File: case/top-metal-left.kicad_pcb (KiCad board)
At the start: 2 copper layers, 134.3 x 93.7 mm, 25 parts, among them SW1 SW_PUSH, SW10 SW_PUSH, SW11 SW_PUSH, SW12 SW_PUSH, SW13 SW_PUSH, SW14 SW_PUSH, SW15 SW_PUSH, SW16 SW_PUSH, SW17 SW_PUSH, SW18 SW_PUSH, SW19 SW_PUSH, SW2 SW_PUSH, SW20 SW_PUSH, SW3 SW_PUSH, SW4 SW_PUSH, SW5 SW_PUSH, SW6 SW_PUSH, SW7 SW_PUSH, SW8 SW_PUSH, SW9 SW_PUSH

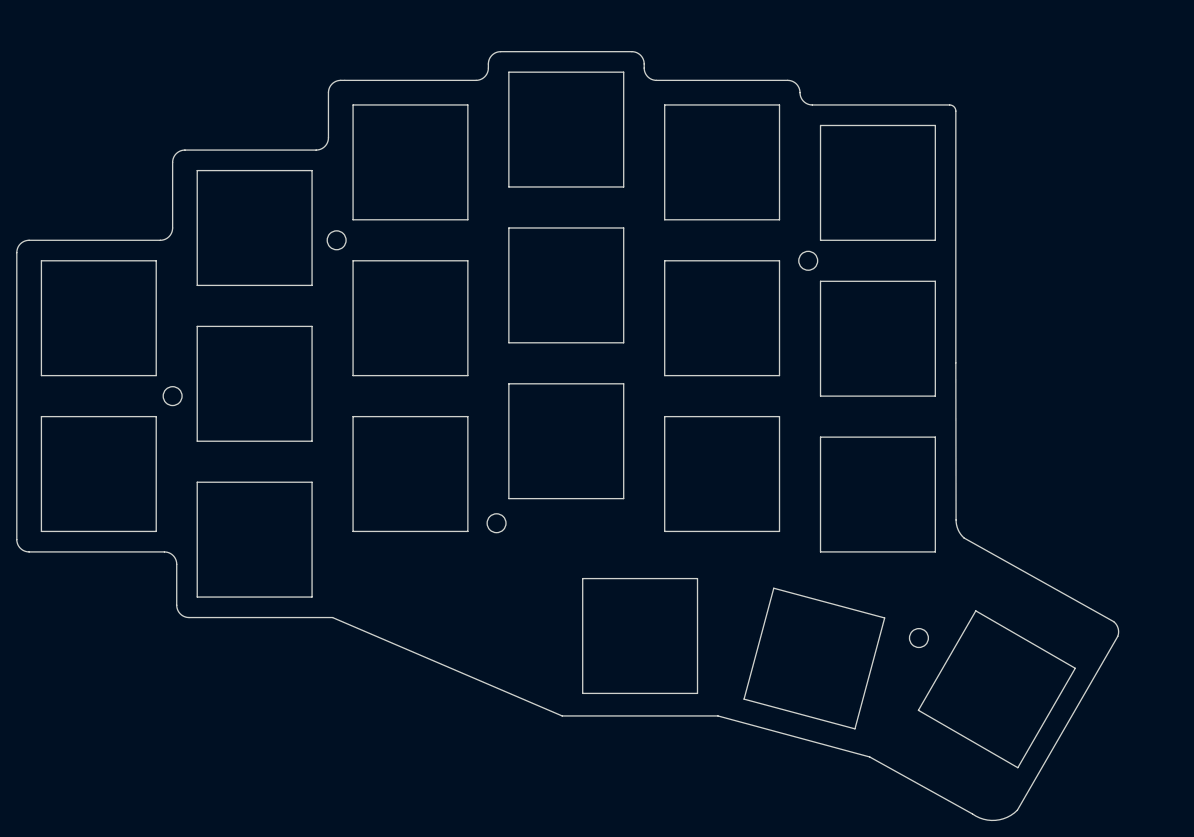
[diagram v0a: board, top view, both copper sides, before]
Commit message: update case files
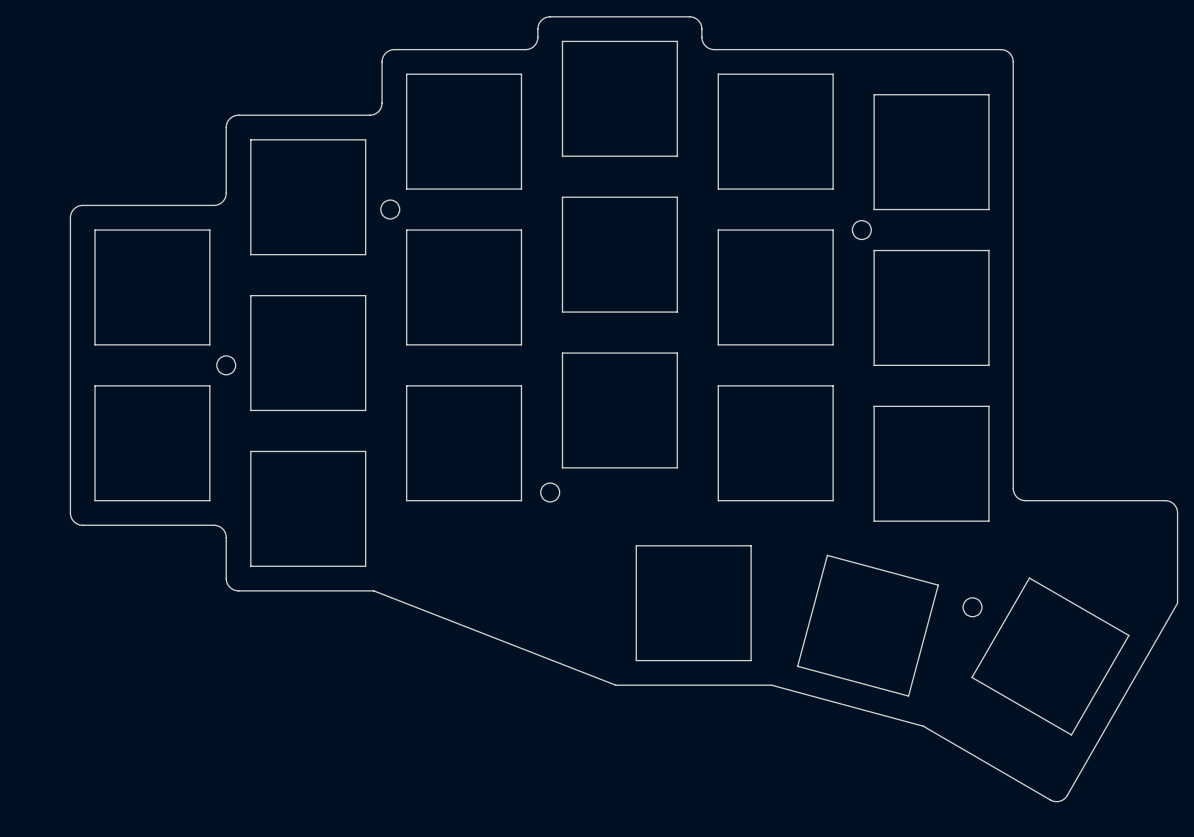
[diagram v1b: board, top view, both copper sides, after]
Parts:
- moved SW18 7.66 mm to (151.0, 118.8)
- moved SW19 7.66 mm to (172.3, 121.5)
- moved SW20 7.66 mm to (194.5, 125.2)
- moved H1 7.54 mm to (114.0, 70.8)
- moved H2 7.54 mm to (185.0, 119.2)
- moved H3 7.54 mm to (94.0, 89.8)
- moved H4 7.54 mm to (133.5, 105.2)
- moved H5 7.54 mm to (171.5, 73.2)
- moved SW1 7.54 mm to (104.0, 69.2)
- moved SW10 7.54 mm to (180.0, 82.8)
- moved SW11 7.54 mm to (104.0, 107.2)
- moved SW12 7.54 mm to (123.0, 99.2)
- moved SW13 7.54 mm to (142.0, 95.2)
- moved SW14 7.54 mm to (161.0, 99.2)
- moved SW15 7.54 mm to (180.0, 101.8)
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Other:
- board size 134.3 x 93.7 mm -> 135 x 95.7 mm
